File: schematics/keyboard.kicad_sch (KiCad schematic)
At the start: 32 parts, among them J2 Mini-DIN-6, Q1 2N7000, Q2 2N7000, Q3 2N7000, Q4 2N7000, Q5 2N7000, U18 74HC14, U19 74HC04, U21 ATF22V10C-7, U22 74HC280, U23 74HC165, U24 74HC595, U25 74HC165, U26 74HC595, U37 74HC245

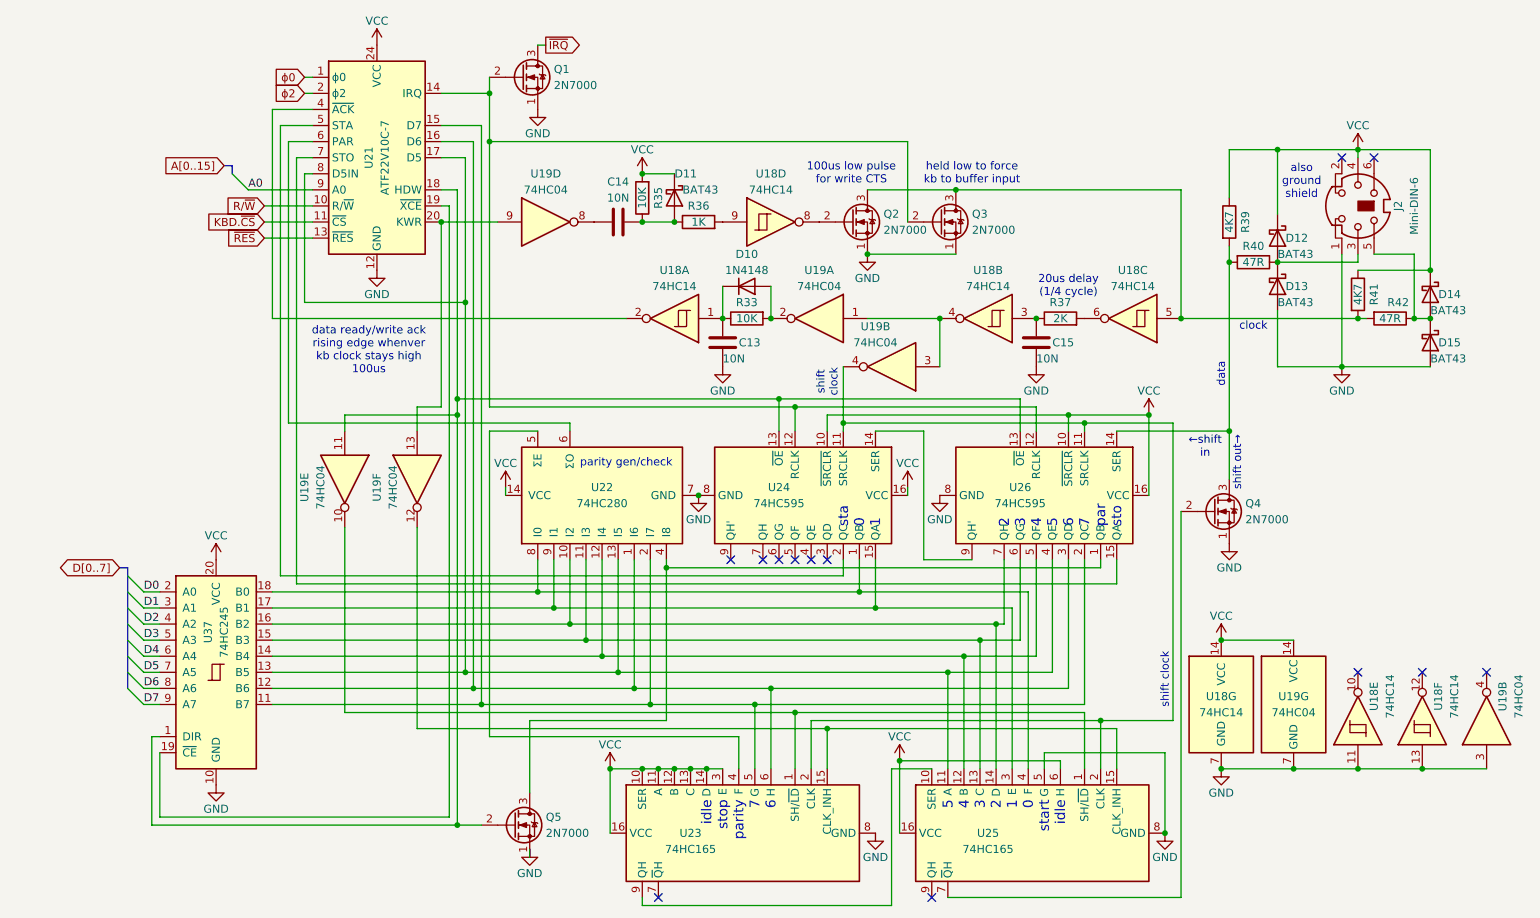
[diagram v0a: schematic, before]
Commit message: done wiring
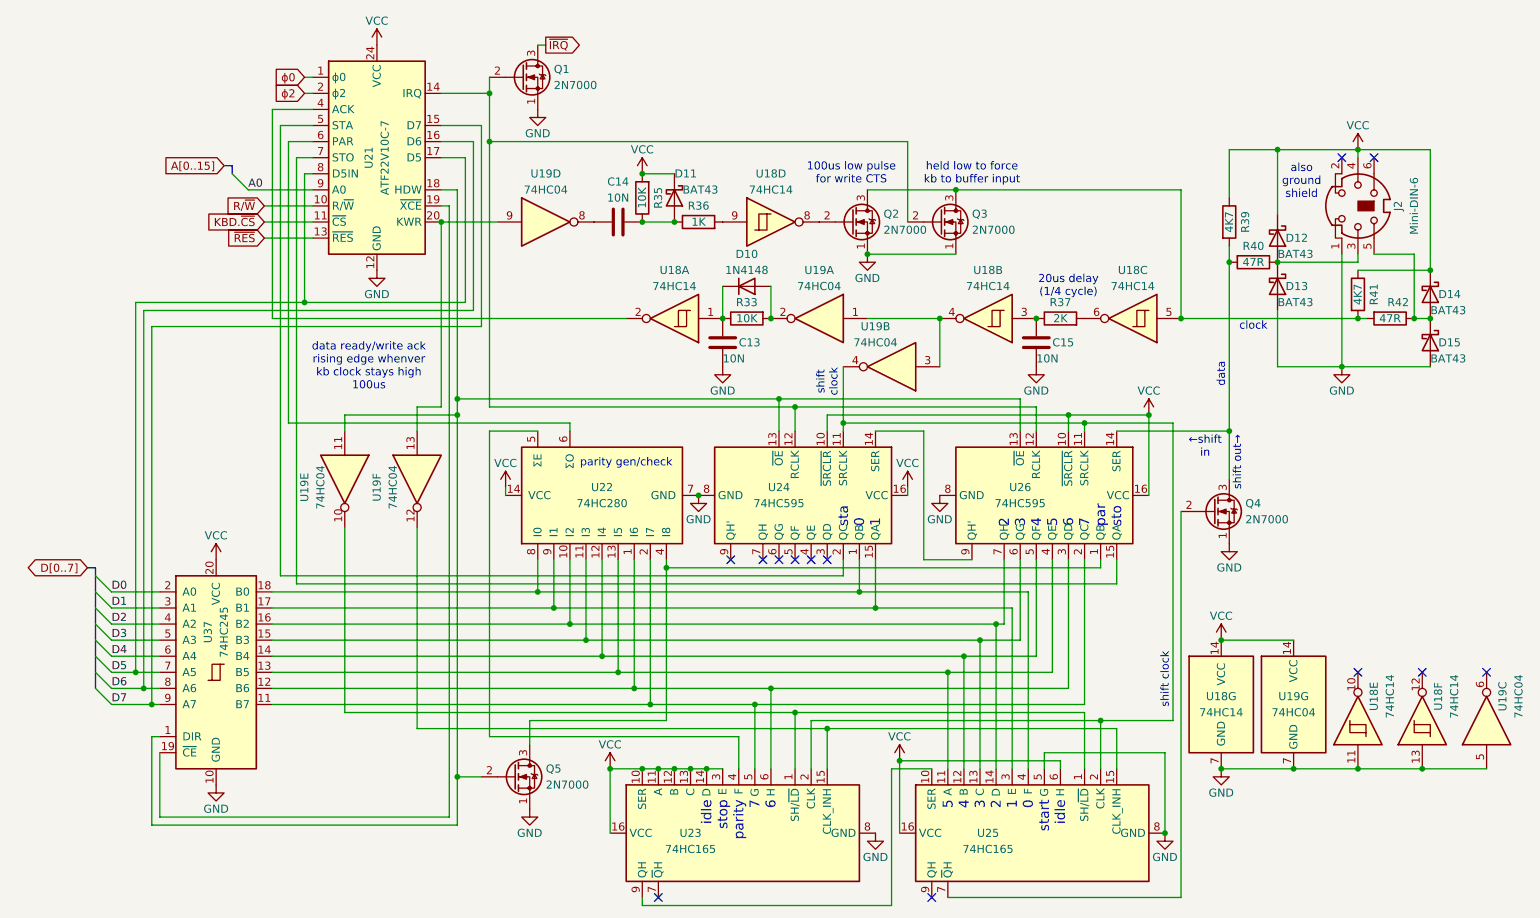
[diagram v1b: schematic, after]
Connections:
- net D5: now also U21.17 (D5), U21.8 (D5IN)
- net D6: now also U21.16 (D6)
- net D7: now also U21.15 (D7)
- net GND: now also U19.5; no longer U19.3
- net at U22.2 (I7), U23.5 (G), U26.2 (QC)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: no longer U21.15 (D7)
- net at U22.1 (I6), U23.6 (H), U26.3 (QD)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: no longer U21.16 (D6)
- net at U22.13 (I5), U25.11 (A), U26.4 (QE)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: no longer U21.17 (D5), U21.8 (D5IN)
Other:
- moved on the sheet: Q5

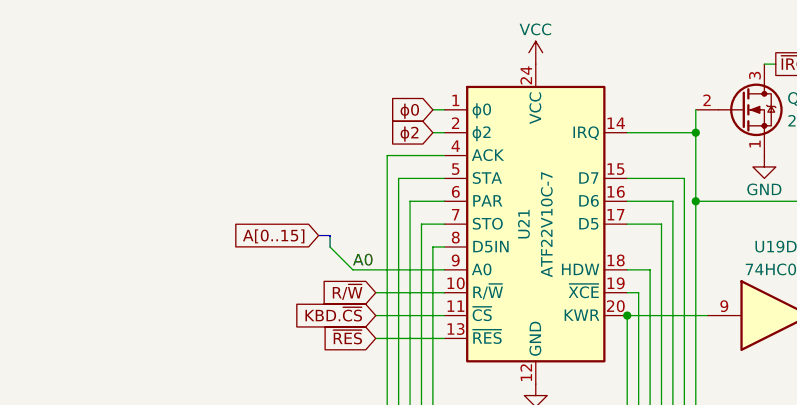
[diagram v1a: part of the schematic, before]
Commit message: clock improvements
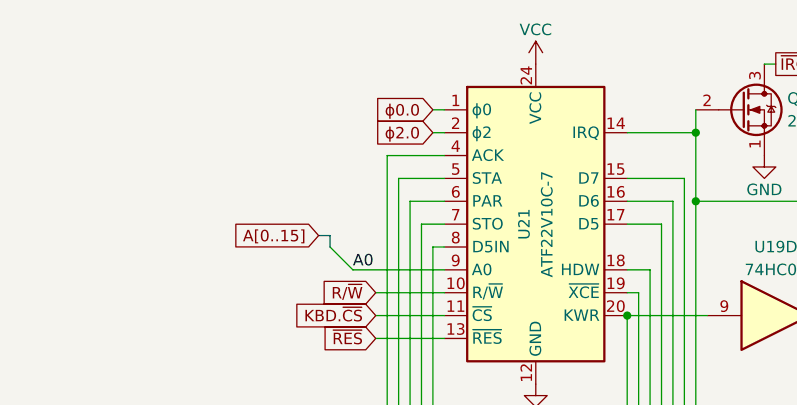
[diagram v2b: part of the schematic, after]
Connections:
- net ϕ0 renamed ϕ0.0
- net ϕ2 renamed ϕ2.0
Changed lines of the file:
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@@
 		)
 	)
-	(global_label "ϕ2"
+	(global_label "ϕ2.0"
 		(shape input)
 		(at 66.04 40.64 180)
@@
 		)
 		(property "Intersheetrefs" "${INTERSHEET_REFS}"
-			(at 60.5148 40.64 0)
+			(at 58.7005 40.64 0)
 			(hide yes)
 			(show_name no)
@@
 		)
 	)
-	(global_label "ϕ0"
+	(global_label "ϕ0.0"
 		(shape input)
 		(at 66.04 38.1 180)
@@
 		)
 		(property "Intersheetrefs" "${INTERSHEET_REFS}"
-			(at 60.5148 38.1 0)
+			(at 58.7005 38.1 0)
 			(hide yes)
 			(show_name no)
